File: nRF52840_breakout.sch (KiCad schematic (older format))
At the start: 32 parts, among them J1 MM8930_2620, U1 nRF52840, Y1 32.768kHz-SIT1533AI-H4-DCC-32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, Y2 32MHz-XRCGB32M000F1H00R0

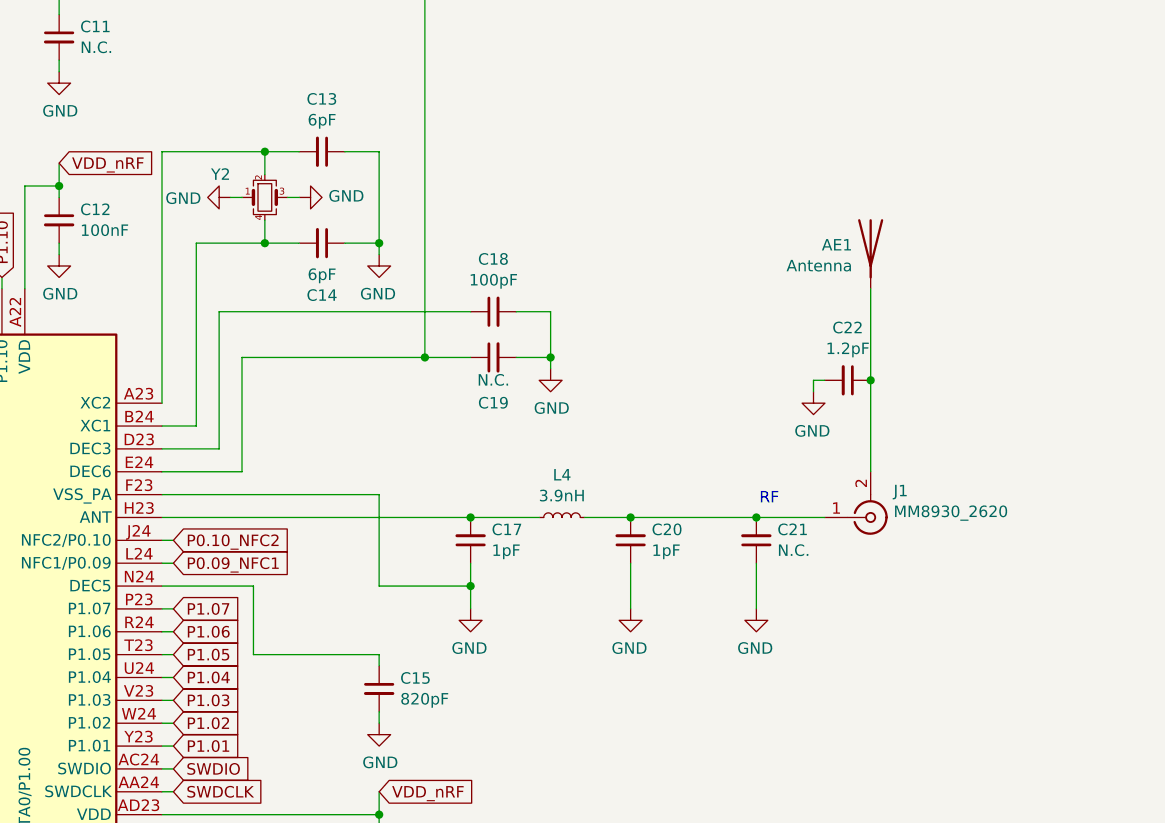
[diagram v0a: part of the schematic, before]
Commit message: path selection/charging/bme680 sensor integration
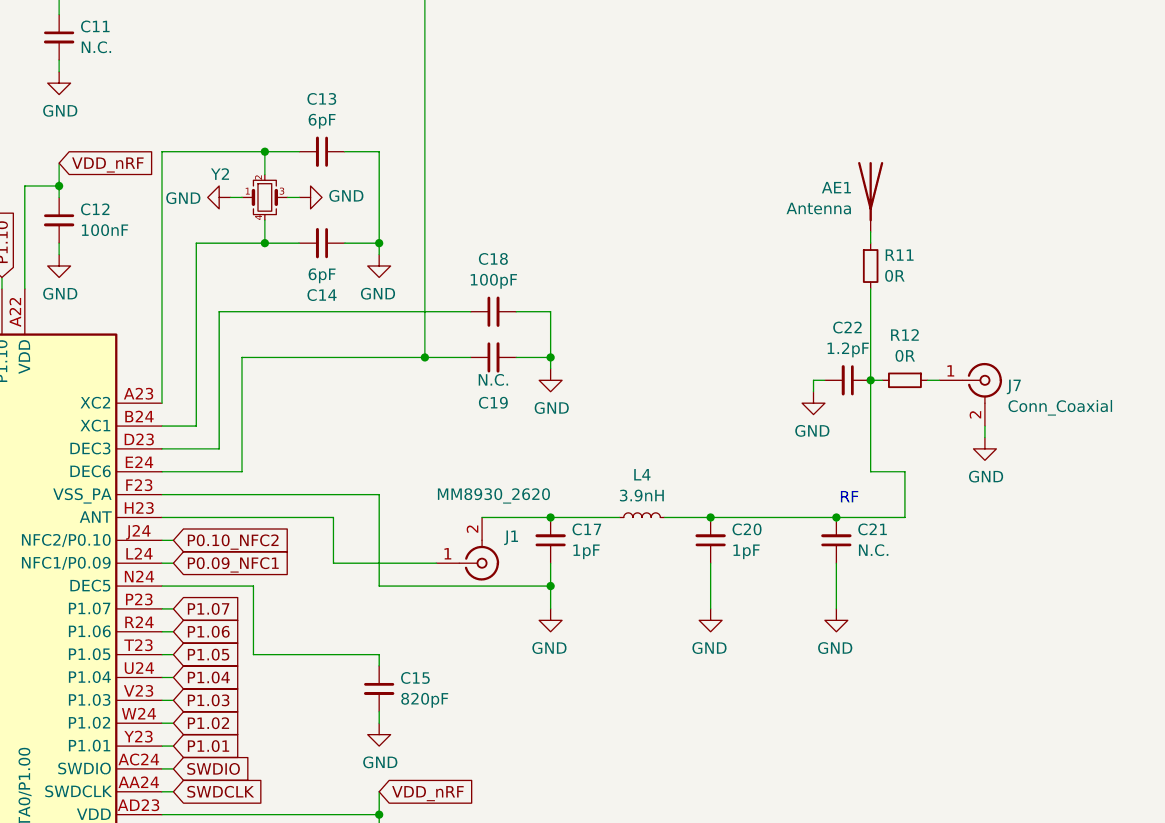
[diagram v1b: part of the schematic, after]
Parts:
- added J7: Conn_Coaxial, custom_footprints:MM8930_2620, symbol Connector:Conn_Coaxial
- added R11, R12: 0R, Resistor_SMD:R_0402_1005Metric, symbol Device:R_Small
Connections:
- net GND: now also J7.2 (Ext)
- net at C20.2, C21.2, L4.1: now also C22.1, R11.2, R12.2; no longer J1.1 (In)
- net at C17.2, L4.2: now also J1.2 (Ext); no longer U1.H23 (ANT)
- new net: AE1.1 (A), R11.1
- new net: J1.1 (In), U1.H23 (ANT)
- new net: J7.1 (In), R12.1
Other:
- moved on the sheet: AE1, C17, C20, C21, J1, L4
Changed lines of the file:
@@
 L Device:L_Small L4
 U 1 1 5C923E84
-P 9000 3250
-F 0 "L4" V 9185 3250 50  0000 C CNN
-F 1 "3.9nH" V 9094 3250 50  0000 C CNN
-F 2 "Inductor_SMD:L_0402_1005Metric" H 9000 3250 50  0001 C CNN
-F 3 "~" H 9000 3250 50  0001 C CNN
-	1    9000 3250
+P 9350 3250
+F 0 "L4" V 9535 3250 50  0000 C CNN
+F 1 "3.9nH" V 9444 3250 50  0000 C CNN
+F 2 "Inductor_SMD:L_0402_1005Metric" H 9350 3250 50  0001 C CNN
+F 3 "~" H 9350 3250 50  0001 C CNN
+	1    9350 3250
 	0    1    -1   0
 $EndComp
@@
 L Device:C_Small C17
 U 1 1 5C923F77
-P 8600 3350
-F 0 "C17" H 8508 3304 50  0000 R CNN
-F 1 "1pF" H 8508 3395 50  0000 R CNN
-F 2 "Capacitor_SMD:C_0402_1005Metric" H 8600 3350 50  0001 C CNN
-F 3 "~" H 8600 3350 50  0001 C CNN
-	1    8600 3350
+P 8950 3350
+F 0 "C17" H 8858 3304 50  0000 R CNN
+F 1 "1pF" H 8858 3395 50  0000 R CNN
+F 2 "Capacitor_SMD:C_0402_1005Metric" H 8950 3350 50  0001 C CNN
+F 3 "~" H 8950 3350 50  0001 C CNN
+	1    8950 3350
 	-1   0    0    1
 $EndComp
@@
 L power:GND #PWR014
 U 1 1 5C924A30
-P 8600 3650
-F 0 "#PWR014" H 8600 3400 50  0001 C CNN
-F 1 "GND" H 8605 3477 50  0000 C CNN
-F 2 "" H 8600 3650 50  0001 C CNN
-F 3 "" H 8600 3650 50  0001 C CNN
-	1    8600 3650
+P 8950 3650
+F 0 "#PWR014" H 8950 3400 50  0001 C CNN
+F 1 "GND" H 8955 3477 50  0000 C CNN
+F 2 "" H 8950 3650 50  0001 C CNN
+F 3 "" H 8950 3650 50  0001 C CNN
+	1    8950 3650
 	-1   0    0    -1
 $EndComp
@@
 L Device:C_Small C20
 U 1 1 5C927D1D
-P 9300 3350
-F 0 "C20" H 9208 3304 50  0000 R CNN
-F 1 "1pF" H 9208 3395 50  0000 R CNN
-F 2 "Capacitor_SMD:C_0402_1005Metric" H 9300 3350 50  0001 C CNN
-F 3 "~" H 9300 3350 50  0001 C CNN
-	1    9300 3350
+P 9650 3350
+F 0 "C20" H 9558 3304 50  0000 R CNN
+F 1 "1pF" H 9558 3395 50  0000 R CNN
+F 2 "Capacitor_SMD:C_0402_1005Metric" H 9650 3350 50  0001 C CNN
+F 3 "~" H 9650 3350 50  0001 C CNN
+	1    9650 3350
 	-1   0    0    1
 $EndComp
 Wire Wire Line
-	9300 3450 9300 3650
-Connection ~ 9300 3250
-Text Notes 9950 3200 2    50   ~ 0
+	9650 3450 9650 3650
+Connection ~ 9650 3250
+Text Notes 10300 3200 2    50   ~ 0
 RF
 $Comp
 L Device:C_Small C21
 U 1 1 5C92A711
-P 9850 3350
-F 0 "C21" H 9758 3304 50  0000 R CNN
-F 1 "N.C." H 9758 3395 50  0000 R CNN
-F 2 "Capacitor_SMD:C_0402_1005Metric" H 9850 3350 50  0001 C CNN
-F 3 "~" H 9850 3350 50  0001 C CNN
-	1    9850 3350
+P 10200 3350
+F 0 "C21" H 10108 3304 50  0000 R CNN
+F 1 "N.C." H 10108 3395 50  0000 R CNN
+F 2 "Capacitor_SMD:C_0402_1005Metric" H 10200 3350 50  0001 C CNN
+F 3 "~" H 10200 3350 50  0001 C CNN
+	1    10200 3350
 	-1   0    0    1
 $EndComp
 Wire Wire Line
-	9850 3250 10150 3250
-Wire Wire Line
-	9850 3450 9850 3650
+	10200 3250 10500 3250
+Wire Wire Line
+	10200 3450 10200 3650
 $Comp
 L Device:C_Small C22
@@
 L Device:Antenna AE1
 U 1 1 5C93430F
-P 10350 2050
-F 0 "AE1" H 10430 2041 50  0000 L CNN
-F 1 "Antenna" H 10430 1950 50  0000 L CNN
-F 2 "RF_Antenna:Texas_SWRA117D_2.4GHz_Right" H 10350 2050 50  0001 C CNN
-F 3 "~" H 10350 2050 50  0001 C CNN
-	1    10350 2050
+P 10350 1800
+F 0 "AE1" H 10430 1791 50  0000 L CNN
+F 1 "Antenna" H 10430 1700 50  0000 L CNN
+F 2 "RF_Antenna:Texas_SWRA117D_2.4GHz_Right" H 10350 1800 50  0001 C CNN
+F 3 "~" H 10350 1800 50  0001 C CNN
+	1    10350 1800
 	-1   0    0    -1
 $EndComp
@@
 L power:GND #PWR016
 U 1 1 5C936B52
-P 9300 3650
-F 0 "#PWR016" H 9300 3400 50  0001 C CNN
-F 1 "GND" H 9305 3477 50  0000 C CNN
-F 2 "" H 9300 3650 50  0001 C CNN
-F 3 "" H 9300 3650 50  0001 C CNN
-	1    9300 3650
+P 9650 3650
+F 0 "#PWR016" H 9650 3400 50  0001 C CNN
+F 1 "GND" H 9655 3477 50  0000 C CNN
+F 2 "" H 9650 3650 50  0001 C CNN
+F 3 "" H 9650 3650 50  0001 C CNN
+	1    9650 3650
 	-1   0    0    -1
 $EndComp
@@
 L power:GND #PWR018
 U 1 1 5C936B97
-P 9850 3650
-F 0 "#PWR018" H 9850 3400 50  0001 C CNN
-F 1 "GND" H 9855 3477 50  0000 C CNN
-F 2 "" H 9850 3650 50  0001 C CNN
-F 3 "" H 9850 3650 50  0001 C CNN
-	1    9850 3650
+P 10200 3650
+F 0 "#PWR018" H 10200 3400 50  0001 C CNN
+F 1 "GND" H 10205 3477 50  0000 C CNN
+F 2 "" H 10200 3650 50  0001 C CNN
+F 3 "" H 10200 3650 50  0001 C CNN
+	1    10200 3650
 	-1   0    0    -1
 $EndComp
@@
 	7300 3450 7250 3450
 Wire Wire Line
-	8600 3450 8600 3550
-Wire Wire Line
-	7250 3250 8600 3250
-Wire Wire Line
-	8600 3250 8900 3250
-Connection ~ 8600 3250
-Wire Wire Line
-	9100 3250 9300 3250
-Wire Wire Line
-	9300 3250 9850 3250
-Connection ~ 9850 3250
+	8950 3450 8950 3550
+Wire Wire Line
+	8950 3250 9250 3250
+Wire Wire Line
+	9450 3250 9650 3250
+Wire Wire Line
+	9650 3250 10200 3250
+Connection ~ 10200 3250
 Wire Wire Line
 	10350 2650 10350 3050
@@
 	10350 2250 10350 2650
 Wire Wire Line
-	8600 3550 8200 3550
-Wire Wire Line
 	8200 3550 8200 3150
 Wire Wire Line
 	8200 3150 7250 3150
-Connection ~ 8600 3550
-Wire Wire Line
-	8600 3550 8600 3650
+Connection ~ 8950 3550
+Wire Wire Line
+	8950 3550 8950 3650
 Wire Wire Line
 	7250 2850 7400 2850
@@
 L Connector:Conn_Coaxial J1
 U 1 1 5CD5A531
-P 10350 3250
-F 0 "J1" H 10450 3134 50  0000 L CNN
-F 1 "MM8930_2620" H 10450 3225 50  0000 L CNN
-F 2 "custom_footprints:MM8930_2620" H 10350 3250 50  0001 C CNN
-F 3 " ~" H 10350 3250 50  0001 C CNN
-	1    10350 3250
+P 8650 3450
+F 0 "J1" H 8750 3334 50  0000 L CNN
+F 1 "MM8930_2620" H 8450 3150 50  0000 L CNN
+F 2 "custom_footprints:MM8930_2620" H 8650 3450 50  0001 C CNN
+F 3 " ~" H 8650 3450 50  0001 C CNN
+	1    8650 3450
 	1    0    0    1
 $EndComp
+$Comp
+L Device:R_Small R11
+U 1 1 5CC69485
+P 10350 2150
+F 0 "R11" H 10409 2196 50  0000 L CNN
+F 1 "0R" H 10409 2105 50  0000 L CNN
+F 2 "Resistor_SMD:R_0402_1005Metric" H 10350 2150 50  0001 C CNN
+F 3 "~" H 10350 2150 50  0001 C CNN
+	1    10350 2150
+	1    0    0    -1
+$EndComp
+Wire Wire Line
+	10350 2000 10350 2050
+$Comp
+L Device:R_Small R12
+U 1 1 5CC72038
+P 10500 2650
+F 0 "R12" V 10304 2650 50  0000 C CNN
+F 1 "0R" V 10395 2650 50  0000 C CNN
+F 2 "Resistor_SMD:R_0402_1005Metric" H 10500 2650 50  0001 C CNN
+F 3 "~" H 10500 2650 50  0001 C CNN
+	1    10500 2650
+	0    1    1    0
+$EndComp
+Wire Wire Line
+	10350 2650 10400 2650
+Wire Wire Line
+	10600 2650 10650 2650
+$Comp
+L Connector:Conn_Coaxial J7
+U 1 1 5CC8403F
+P 10850 2650
+F 0 "J7" H 10949 2626 50  0000 L CNN
+F 1 "Conn_Coaxial" H 10949 2535 50  0000 L CNN
+F 2 "custom_footprints:MM8930_2620" H 10850 2650 50  0001 C CNN
+F 3 " ~" H 10850 2650 50  0001 C CNN
+	1    10850 2650
+	1    0    0    -1
+$EndComp
+$Comp
+L power:GND #PWR023
+U 1 1 5CC84745
+P 10850 2900
+F 0 "#PWR023" H 10850 2650 50  0001 C CNN
+F 1 "GND" H 10855 2727 50  0000 C CNN
+F 2 "" H 10850 2900 50  0001 C CNN
+F 3 "" H 10850 2900 50  0001 C CNN
+	1    10850 2900
+	1    0    0    -1
+$EndComp
+Wire Wire Line
+	10850 2850 10850 2900
+Wire Wire Line
+	7250 3250 8000 3250
+Wire Wire Line
+	8000 3250 8000 3450
+Wire Wire Line
+	8000 3450 8450 3450
+Wire Wire Line
+	8200 3550 8950 3550
+Wire Wire Line
+	8650 3250 8950 3250
+Connection ~ 8950 3250
+Wire Wire Line
+	10500 3250 10500 3050
+Wire Wire Line
+	10500 3050 10350 3050
 $EndSCHEMATC
